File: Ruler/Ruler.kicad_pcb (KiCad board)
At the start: 2 copper layers, 100 x 25 mm, 20 parts, among them Q1 NPN, Q2 NPN, Q3 NPN, Q4 NPN, U1 IR2302, U3 STM32F303K8Tx

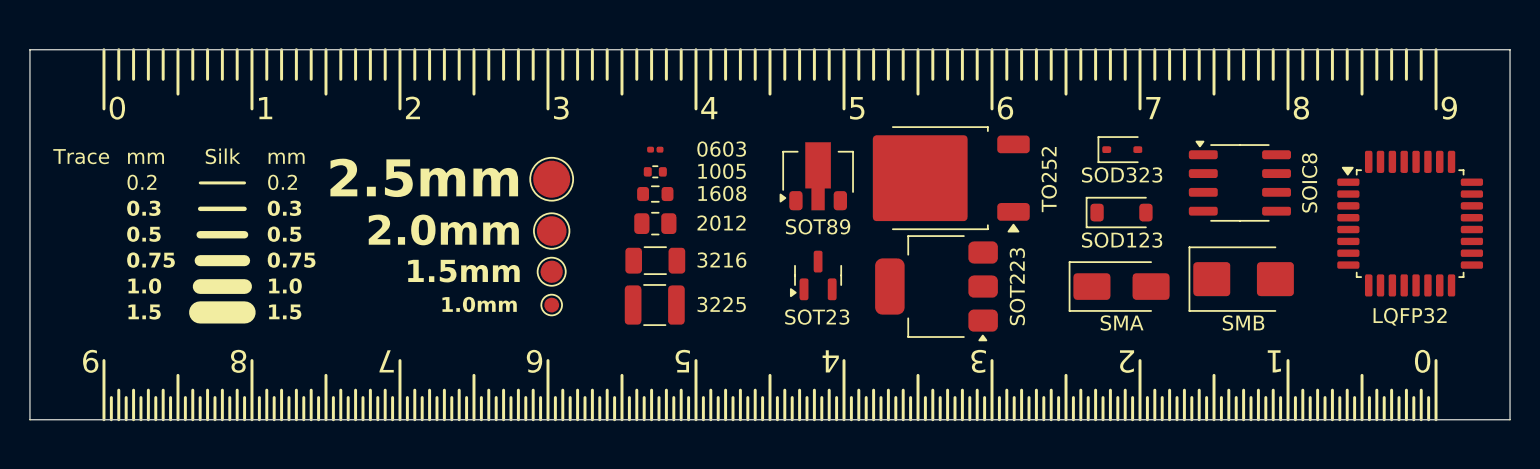
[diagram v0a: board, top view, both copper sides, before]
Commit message: 裏面途中
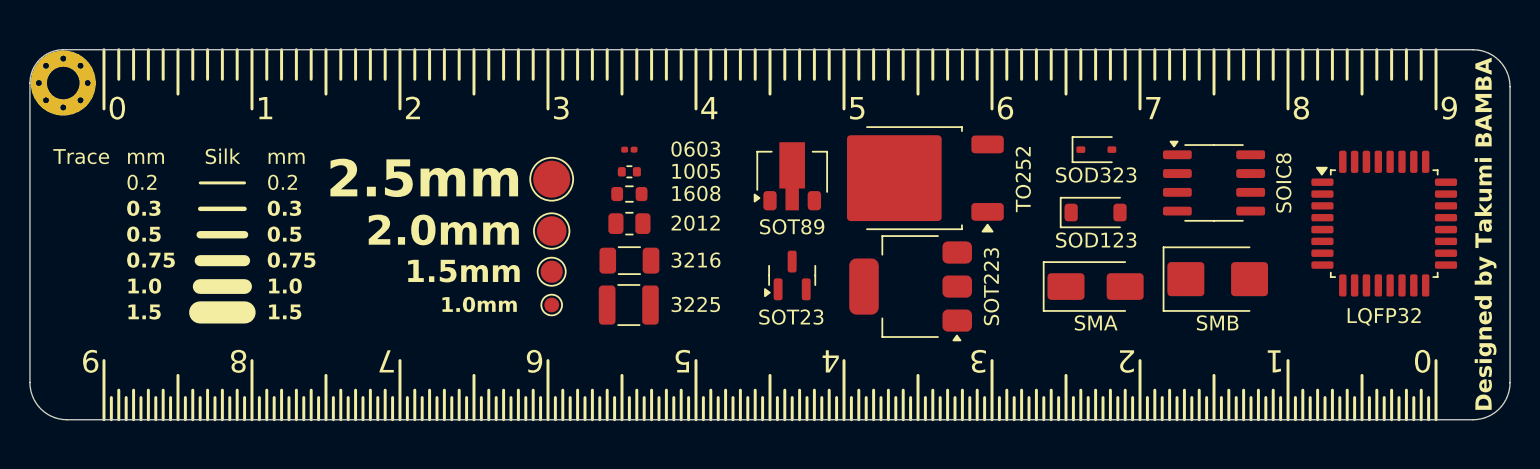
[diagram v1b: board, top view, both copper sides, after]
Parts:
- removed U3: STM32F303K8Tx, Package_QFP:LQFP-32_7x7mm_P0.8mm
- added H1: MountingHole, MountingHole:MountingHole_2.2mm_M2_Pad_Via, F.Cu at (102.2, 102.2)
- added U2: STM32F303K8Tx, Package_QFP:LQFP-32_7x7mm_P0.8mm, F.Cu at (191.5, 111.8)
- moved D1 1.75 mm to (172.0, 111.0)
- moved D2 1.75 mm to (172.1, 106.8)
- moved D3 1.75 mm to (172.0, 116.0)
- moved D4 1.75 mm to (180.2, 115.5)
- moved Q1 1.75 mm to (151.5, 115.2)
- moved Q2 1.75 mm to (159.5, 116.0)
- moved Q3 1.75 mm to (151.5, 108.2)
- moved Q4 1.75 mm to (159.7, 108.7)
- moved R1 1.75 mm to (140.5, 106.8)
- moved R2 1.75 mm to (140.5, 108.2)
- moved R3 1.75 mm to (140.5, 109.8)
- moved R4 1.75 mm to (140.5, 111.8)
- moved R5 1.75 mm to (140.5, 114.2)
- moved R6 1.75 mm to (140.5, 117.2)
- moved U1 1.75 mm to (180.0, 109.0)
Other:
- outline, holes or cut-outs redrawn
- board text added: "B"
- board text added: "C"
- board text added: "D"
- board text added: "Designed by Takumi BAMBA"
- board text added: "Diode"
- board text added: "E"
- board text added: "G"
- board text added: "LED"
- board text added: "MOSFET"
- board text added: "NPN"
- board text added: "Nch"
- board text added: "Normal"
- board text added: "PNP"
- board text added: "Pch"
- board text added: "Photo"
- board text added: "S"
- board text added: "Schottky"
- board text added: "Transistor"
- board text added: "Varactor"

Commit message: 発注した
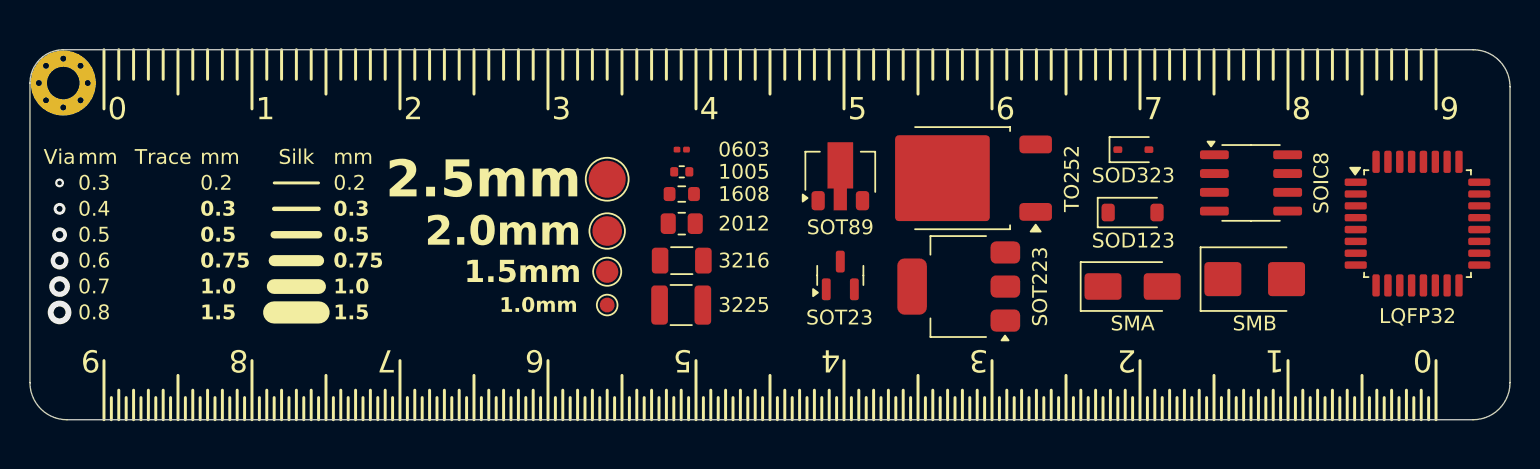
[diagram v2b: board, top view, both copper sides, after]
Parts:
- added G***: LOGO, 0MyLibrary:JLCPCB_40mm, B.Cu at (172.6, 115.5)
- added G***: LOGO, 0MyLibrary:KiCad_20mm, B.Cu at (182.6, 108.2)
- moved TP1 3.75 mm to (139.0, 117.2)
- moved TP2 3.75 mm to (139.0, 115.0)
- moved TP3 3.75 mm to (139.0, 112.2)
- moved TP4 3.75 mm to (139.0, 108.8)
- moved R1 3.54 mm to (144.0, 106.8)
- moved R2 3.54 mm to (144.0, 108.2)
- moved R3 3.54 mm to (144.0, 109.8)
- moved R4 3.54 mm to (144.0, 111.8)
- moved R5 3.54 mm to (144.0, 114.2)
- moved R6 3.54 mm to (144.0, 117.2)
- moved Q1 3.25 mm to (154.8, 115.2)
- moved Q2 3.25 mm to (162.8, 116.0)
- moved Q3 3.25 mm to (154.8, 108.2)
- moved Q4 3.25 mm to (162.9, 108.7)
- moved D1 2.50 mm to (174.5, 111.0)
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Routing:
- net (no net): vias 0 -> 6
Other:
- board text added: "0.4"
- board text added: "0.6"
- board text added: "0.7"
- board text added: "0.8"
- board text added: "Takumi BAMBA"
- board text added: "Via"
- board text removed: "Designed by Takumi BAMBA"
